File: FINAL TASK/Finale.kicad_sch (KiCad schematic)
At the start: 31 parts, among them J1 Conn_01x04_Pin, J2 Conn_01x04_Pin, P1 USB_C_Plug, SW1 RESET, SW2 SW_SPDT, U1 STM32F103C8T6, U2 AS5048B, U3 AS5048B, U4 AS5048B, U5 AS5048B, U6 AMS1117-3.3, Y1 16MHz

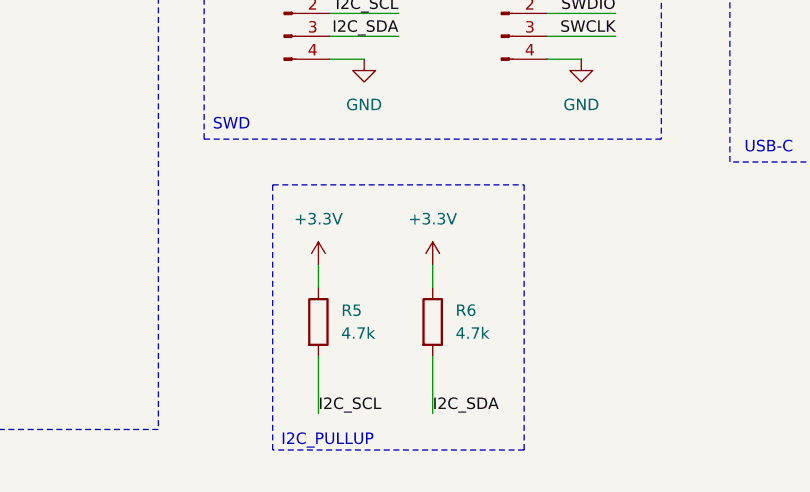
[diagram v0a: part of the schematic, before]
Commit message: Done
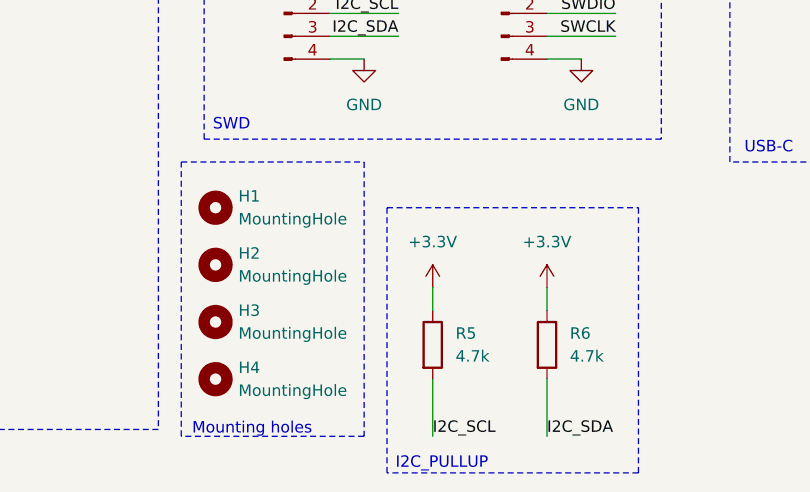
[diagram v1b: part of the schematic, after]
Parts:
- added H1, H2, H3, H4: MountingHole, MountingHole:MountingHole_2.1mm, symbol Mechanical:MountingHole
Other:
- note added: "Mounting holes"
- moved on the sheet: R5, R6
